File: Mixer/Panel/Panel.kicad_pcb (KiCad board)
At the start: 2 copper layers, 70.8 x 128.5 mm, 0 parts

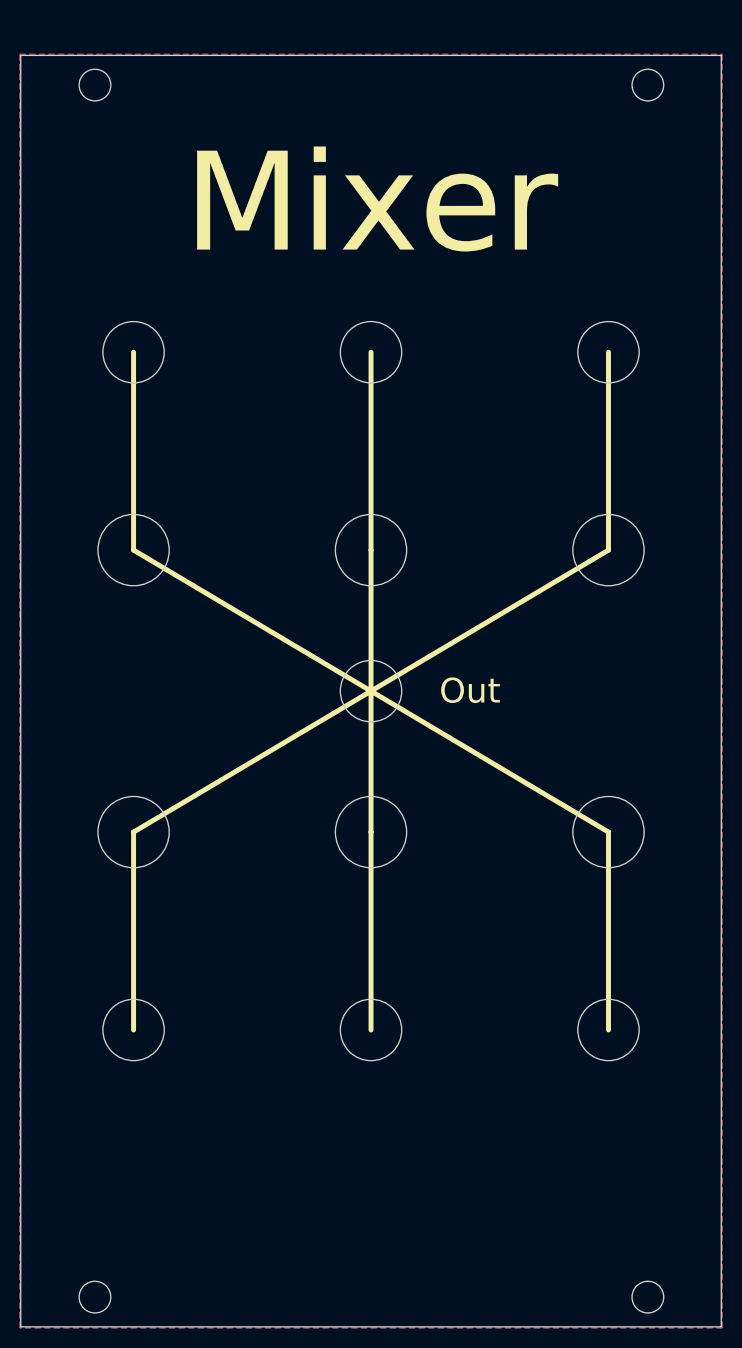
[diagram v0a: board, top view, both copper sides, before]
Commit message: Finish main set of revisions
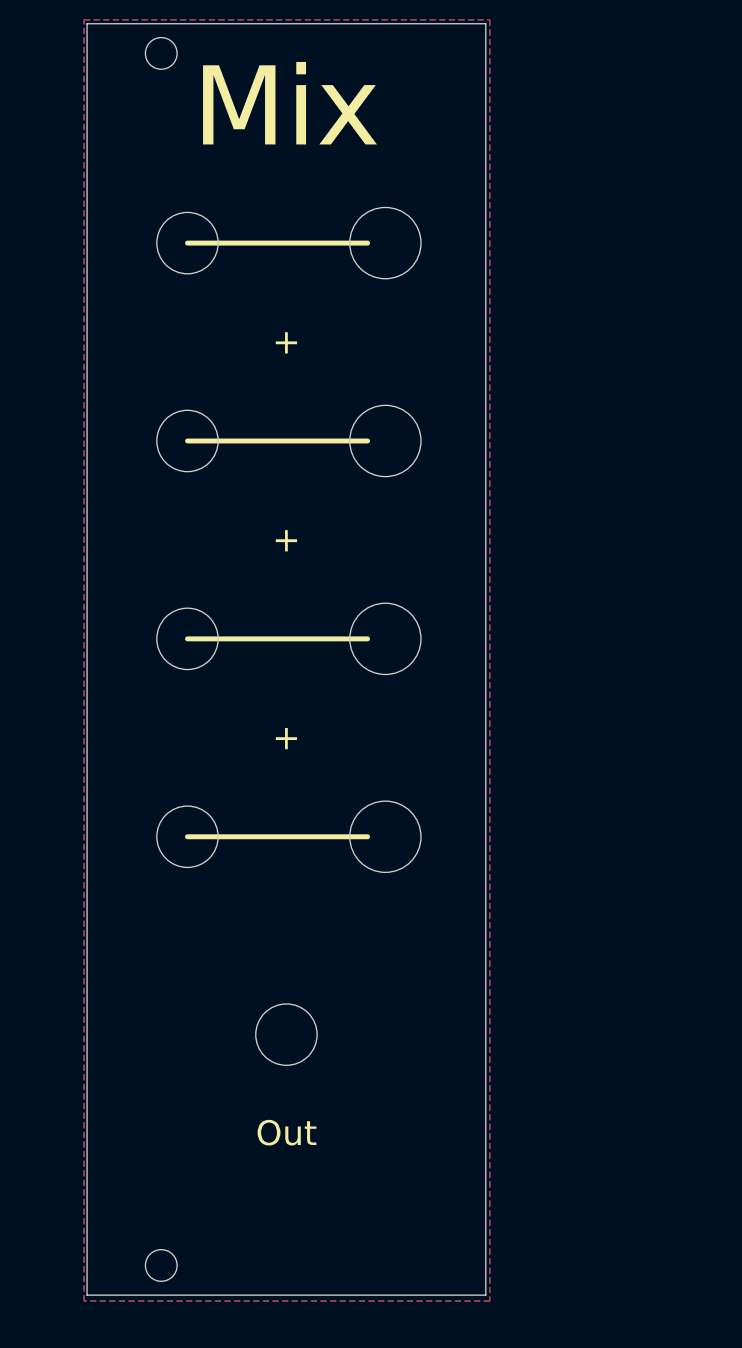
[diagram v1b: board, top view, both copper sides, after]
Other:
- board size 70.8 x 128.5 mm -> 40.3 x 128.5 mm
- board text added: "+"
- board text added: "Mix"
- board text removed: "Mixer"
